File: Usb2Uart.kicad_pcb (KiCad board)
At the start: 2 copper layers, 46.2 x 16.2 mm, 46 parts, among them Q1 DVIUC6-4SC6, U1 DLW21SN900SQ2

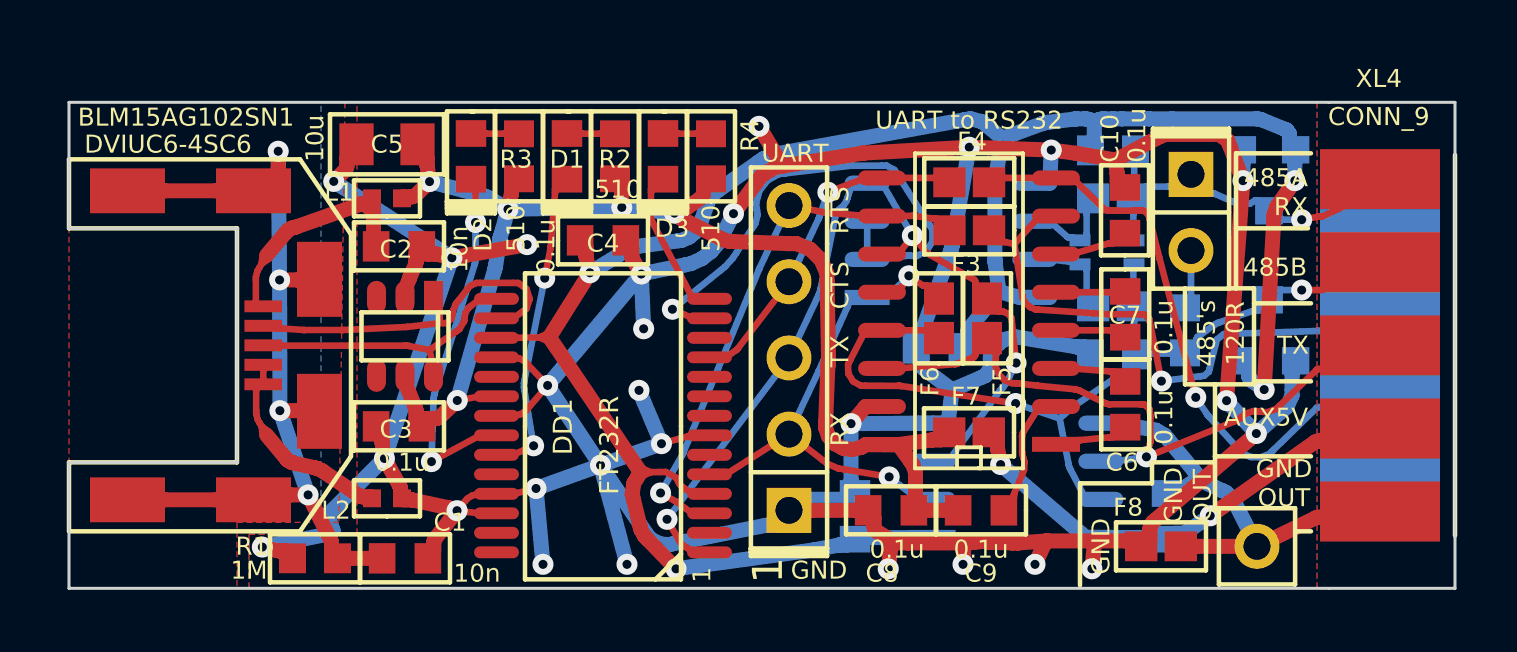
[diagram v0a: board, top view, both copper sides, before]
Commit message: toporrrrrr
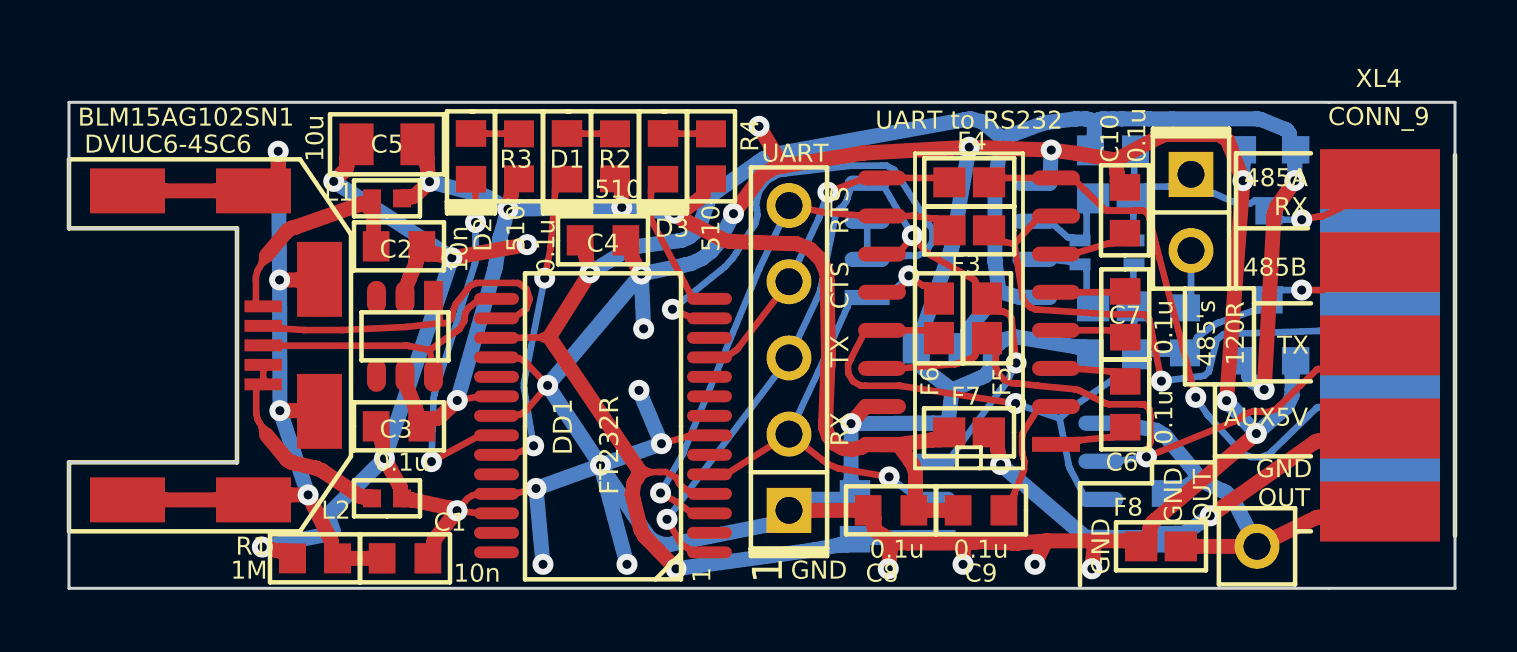
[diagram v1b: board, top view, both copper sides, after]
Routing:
- net /RTS: track 19.6 -> 29.3 mm, vias 1 -> 2
- net /CTS: track 20.0 -> 10.2 mm, vias 1 -> 0
- net /Aux5V: track 15.9 -> 12.1 mm
- net /RS485B_RX: track 30.3 -> 34.1 mm
- removed copper zone on F.Cu, net /SHLD
- removed copper zone on B.Cu, net GND
- removed copper zone on F.Cu, net GND
